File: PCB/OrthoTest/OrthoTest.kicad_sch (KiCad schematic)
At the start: 121 parts, among them SW1 SW_Push, SW10 SW_Push, SW11 SW_Push, SW12 SW_Push, SW13 SW_Push, SW14 SW_Push, SW15 SW_Push, SW16 SW_Push, SW17 SW_Push, SW18 SW_Push, SW19 SW_Push, SW2 SW_Push, SW20 SW_Push, SW21 SW_Push, SW22 SW_Push, SW23 SW_Push, SW24 SW_Push, SW25 SW_Push, SW26 SW_Push, SW27 SW_Push, SW28 SW_Push, SW29 SW_Push, SW3 SW_Push, SW30 SW_Push, SW31 SW_Push, SW32 SW_Push, SW33 SW_Push, SW34 SW_Push, SW35 SW_Push, SW36 SW_Push, SW37 SW_Push, SW38 SW_Push, SW39 SW_Push, SW4 SW_Push, SW40 SW_Push, SW41 SW_Push, SW42 SW_Push, SW43 SW_Push, SW44 SW_Push, SW45 SW_Push, SW46 SW_Push, SW47 SW_Push, SW48 SW_Push, SW49 SW_Push, SW5 SW_Push, SW50 SW_Push, SW51 SW_Push, SW52 SW_Push, SW53 SW_Push, SW54 SW_Push, SW55 SW_Push, SW56 SW_Push, SW57 SW_Push, SW58 SW_Push, SW59 SW_Push, SW6 SW_Push, SW60 SW_Push, SW7 SW_Push, SW8 SW_Push, SW9 SW_Push

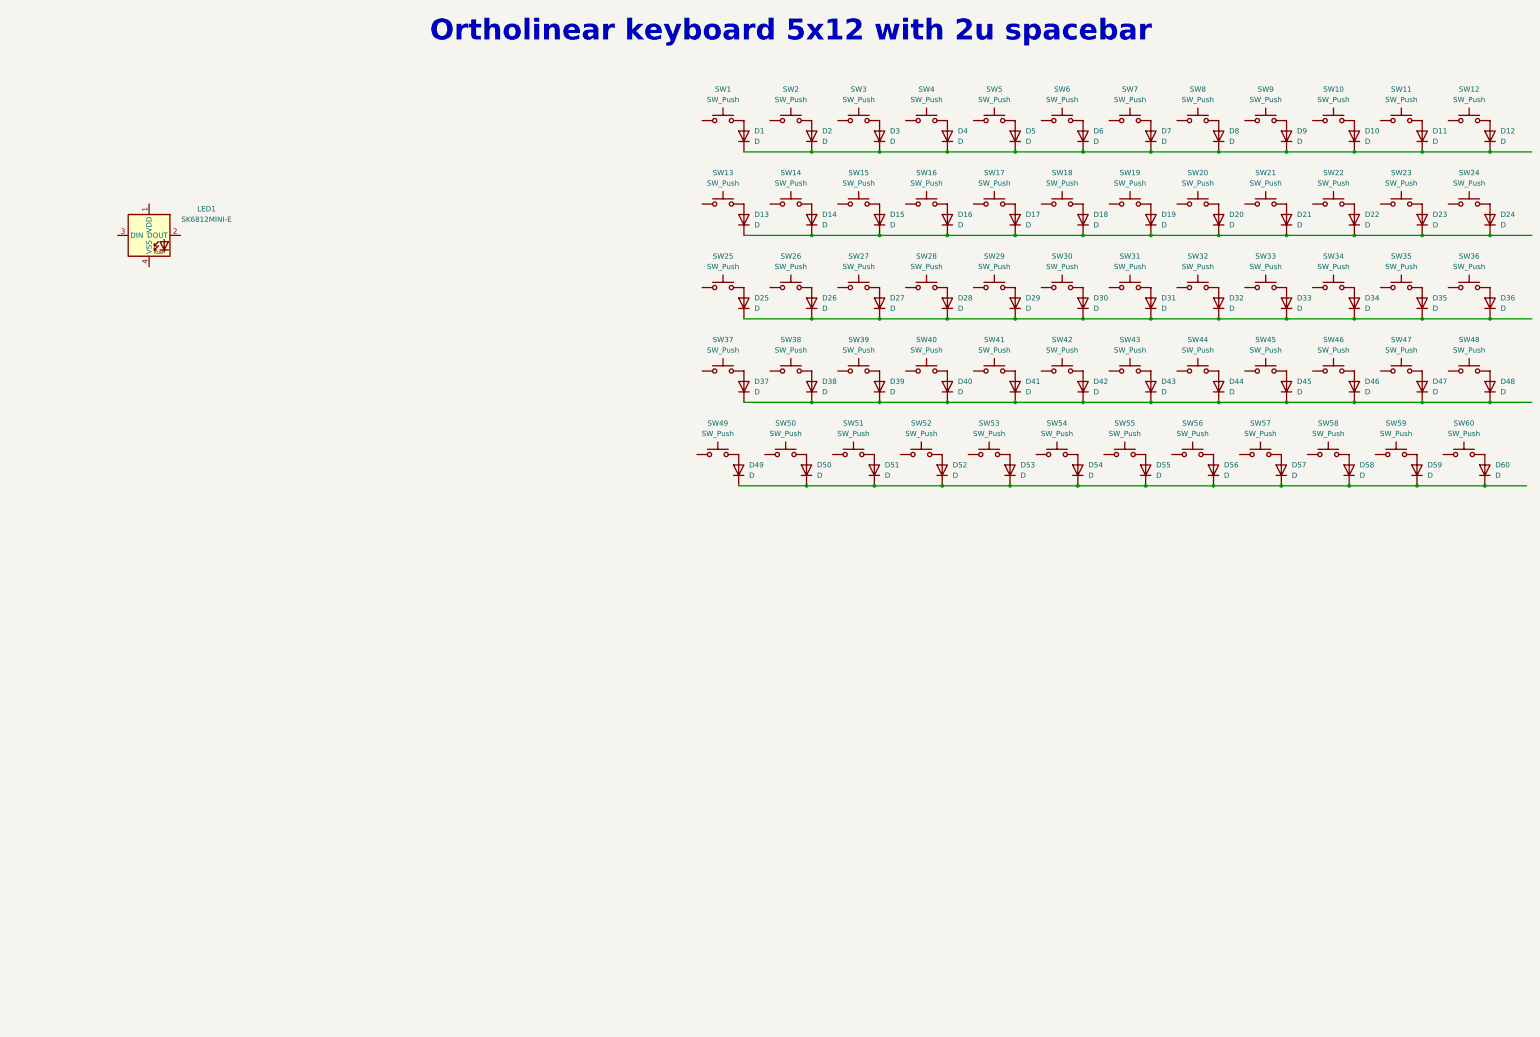
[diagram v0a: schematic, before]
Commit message: worked on it a lil
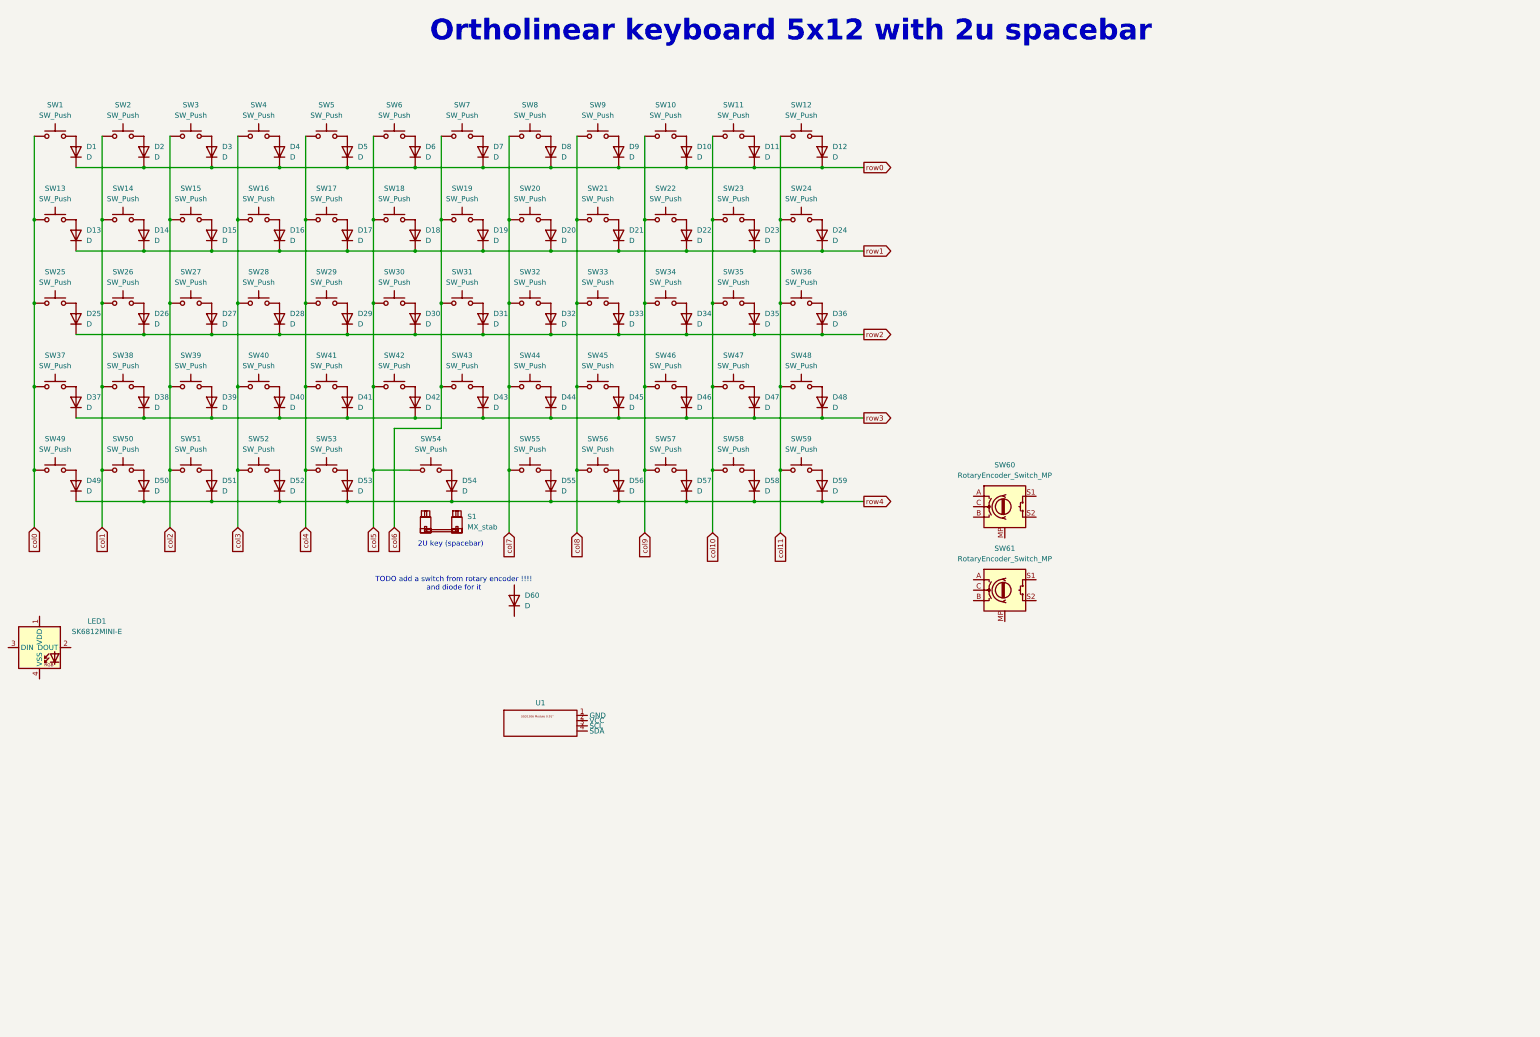
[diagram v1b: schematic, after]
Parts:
- removed SW60: SW_Push, MyKeebLib:SW_Redragon_LowProfile_PCB_1.00u, symbol Switch:SW_Push
- added S1: MX_stab, PCM_marbastlib-mx:STAB_MX_2u, symbol PCM_marbastlib-mx:MX_stab
- added SW60, SW61: RotaryEncoder_Switch_MP, Rotary_Encoder:RotaryEncoder_Alps_EC11E-Switch_Vertical_H20mm, symbol Device:RotaryEncoder_Switch_MP
- added U1: ~, MyKeebLib:SSD1306-0.91-OLED-4pin-128x32, symbol MySymbols:ssd1306
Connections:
- net row1: now reaches D13.1 (K), D14.1 (K), D15.1 (K), D16.1 (K), D17.1 (K), D18.1 (K), D19.1 (K), D20.1 (K), D21.1 (K), D22.1 (K), D23.1 (K), D24.1 (K)
- net row2: now reaches D25.1 (K), D26.1 (K), D27.1 (K), D28.1 (K), D29.1 (K), D30.1 (K), D31.1 (K), D32.1 (K), D33.1 (K), D34.1 (K), D35.1 (K), D36.1 (K)
- net row0: now reaches D1.1 (K), D10.1 (K), D11.1 (K), D12.1 (K), D2.1 (K), D3.1 (K), D4.1 (K), D5.1 (K), D6.1 (K), D7.1 (K), D8.1 (K), D9.1 (K)
- net col10: now reaches SW47.1
- net col10: now also SW11.1, SW23.1, SW35.1, SW58.1
- net row3: now reaches D37.1 (K), D38.1 (K), D39.1 (K), D40.1 (K), D41.1 (K), D42.1 (K), D43.1 (K), D44.1 (K), D45.1 (K), D46.1 (K), D47.1 (K), D48.1 (K)
- net col2: now reaches SW3.1
- net col2: now also SW15.1, SW27.1, SW39.1, SW51.1
- net col0: now reaches SW25.1
- net col0: now also SW1.1, SW13.1, SW37.1, SW49.1
- net col7: now reaches SW8.1
- net col7: now also SW20.1, SW32.1, SW44.1, SW55.1
- net col1: now reaches SW50.1
- net col1: now also SW14.1, SW2.1, SW26.1, SW38.1
- net col5: now reaches SW30.1
- net col5: now also SW18.1, SW42.1, SW54.1, SW6.1
- net col4: now reaches SW41.1
- net col4: now also SW17.1, SW29.1, SW5.1, SW53.1
- net row4: now reaches D49.1 (K), D50.1 (K), D51.1 (K), D52.1 (K), D53.1 (K), D54.1 (K), D55.1 (K), D56.1 (K), D57.1 (K), D58.1 (K), D59.1 (K)
- net row4: no longer D60.1 (K)
- net col3: now reaches SW52.1
- net col3: now also SW16.1, SW28.1, SW4.1, SW40.1
- net col9: now reaches SW22.1
- net col9: now also SW10.1, SW34.1, SW46.1, SW57.1
- net col11: now reaches SW24.1
- net col11: now also SW12.1, SW36.1, SW48.1, SW59.1
- net col8: now reaches SW21.1
- net col8: now also SW33.1, SW45.1, SW56.1, SW9.1
- net col6: now reaches SW19.1
- net col6: now also SW31.1, SW43.1, SW7.1
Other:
- note added: "2U key (spacebar)"
- note added: "TODO add a switch from rotary encoder !!!! and diode for it"
- moved on the sheet: D1, D10, D11, D12, D13, D14, D15, D16, D17, D18, D19, D2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

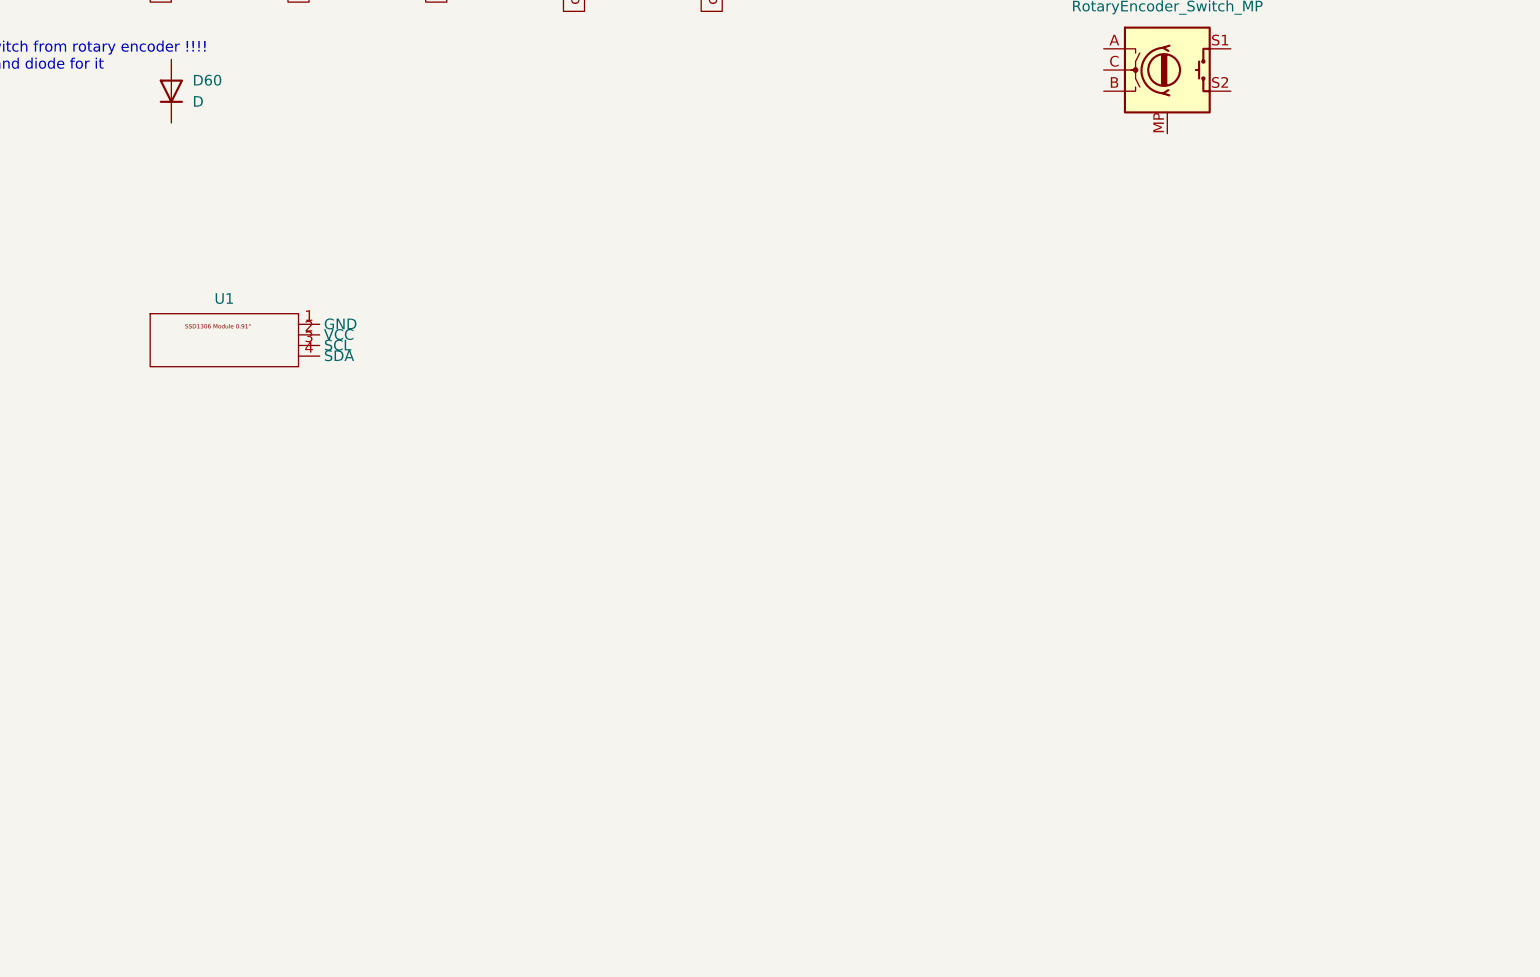
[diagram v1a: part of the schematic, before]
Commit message: worked a lil on it
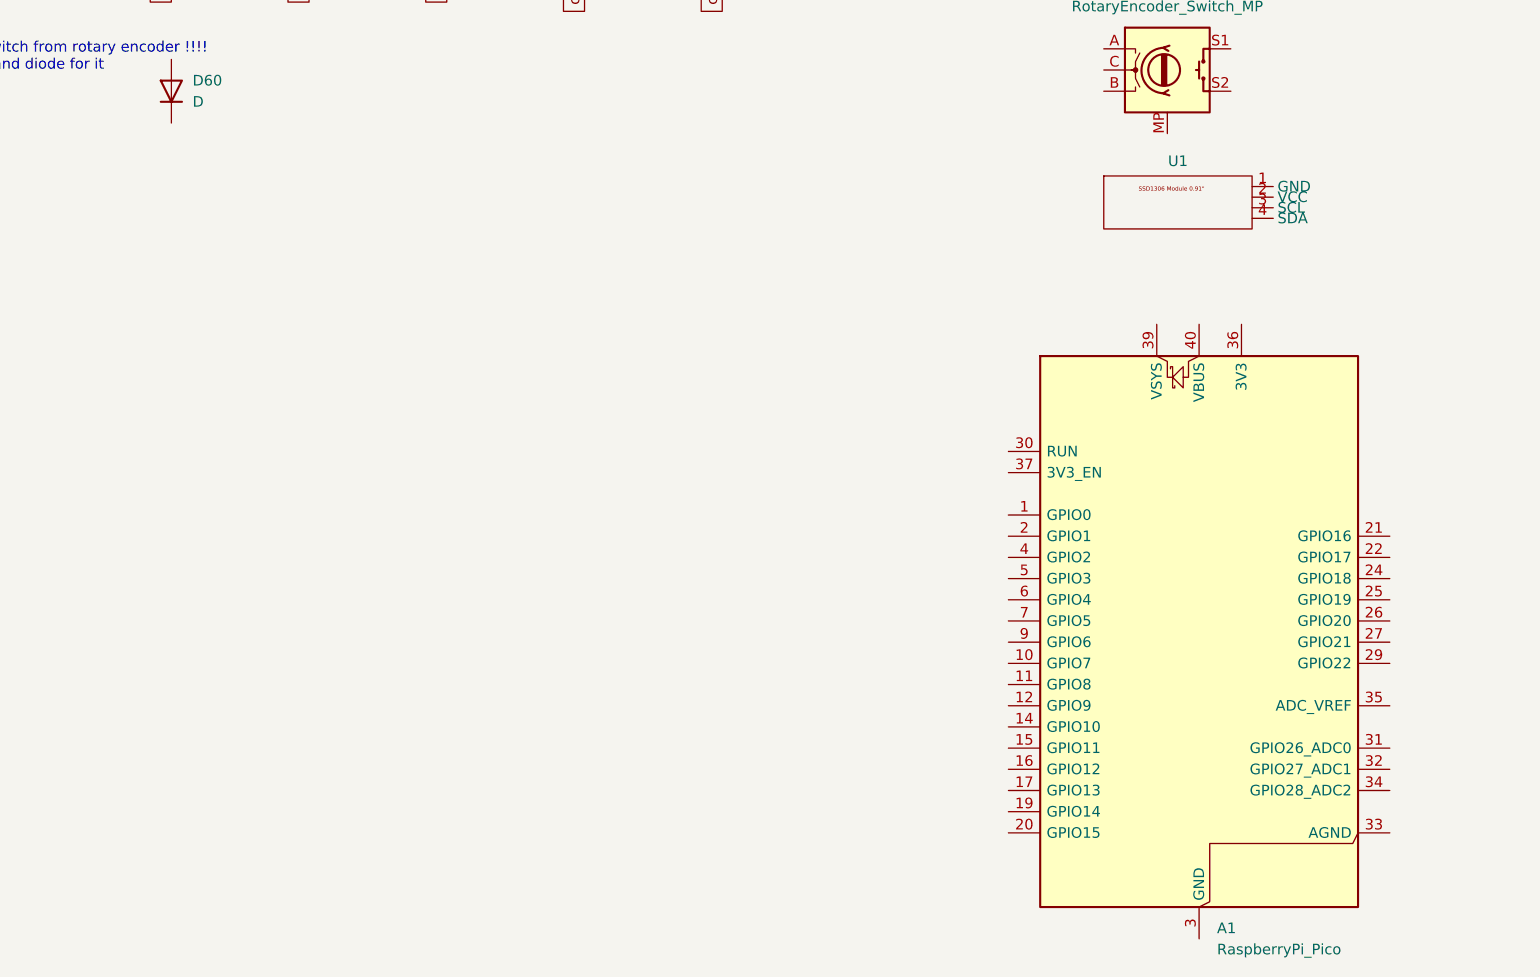
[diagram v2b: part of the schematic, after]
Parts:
- added A1: RaspberryPi_Pico, Module:RaspberryPi_Pico_Common_SMD, symbol MCU_Module:RaspberryPi_Pico
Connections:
- new net: A1.13 (GND), A1.18 (GND), A1.23 (GND), A1.28 (GND), A1.3 (GND), A1.38 (GND), A1.8 (GND)
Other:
- moved on the sheet: U1
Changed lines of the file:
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@@
 	(symbol
 		(lib_id "MySymbols:ssd1306")
-		(at 151.13 189.23 0)
+		(at 265.43 172.72 0)
 		(unit 1)
 		(exclude_from_sim no)
@@
 		(dnp no)
 		(property "Reference" "U1"
-			(at 151.13 188.722 0)
+			(at 265.43 172.212 0)
 			(effects
 				(font
@@
 		)
 		(property "Value" "~"
-			(at 152.4 189.23 0)
+			(at 266.7 172.72 0)
 			(effects
 				(font
@@
 		)
 		(property "Footprint" "MyKeebLib:SSD1306-0.91-OLED-4pin-128x32"
-			(at 151.13 189.23 0)
+			(at 265.43 172.72 0)
 			(effects
 				(font
@@
 		)
 		(property "Datasheet" ""
-			(at 151.13 189.23 0)
+			(at 265.43 172.72 0)
 			(effects
 				(font
@@
 		)
 		(property "Description" ""
-			(at 151.13 189.23 0)
+			(at 265.43 172.72 0)
 			(effects
 				(font
@@
 					(unit 1)
 				)
+			)
+		)
+	)
+	(symbol
+		(lib_id "MCU_Module:RaspberryPi_Pico")
+		(at 267.97 229.87 0)
+		(unit 1)
+		(exclude_from_sim no)
+		(in_bom yes)
+		(on_board yes)
+		(dnp no)
+		(fields_autoplaced yes)
+		(property "Reference" "A1"
+			(at 270.1133 264.16 0)
+			(effects
+				(font
+					(size 1.27 1.27)
+				)
+				(justify left)
+			)
+		)
+		(property "Value" "RaspberryPi_Pico"
+			(at 270.1133 266.7 0)
+			(effects
+				(font
+					(size 1.27 1.27)
+				)
+				(justify left)
+			)
+		)
+		(property "Footprint" "Module:RaspberryPi_Pico_Common_SMD"
+			(at 267.97 276.86 0)
+			(effects
+				(font
+					(size 1.27 1.27)
+				)
+				(hide yes)
+			)
+		)
+		(property "Datasheet" "https://datasheets.raspberrypi.com/pico/pico-datasheet.pdf"
+			(at 267.97 279.4 0)
+			(effects
+				(font
+					(size 1.27 1.27)
+				)
+				(hide yes)
+			)
+		)
+		(property "Description" "Versatile and inexpensive microcontroller module powered by RP2040 dual-core Arm Cortex-M0+ processor up to 133 MHz, 264kB SRAM, 2MB QSPI flash; also supports Raspberry Pi Pico 2"
+			(at 267.97 281.94 0)
+			(effects
+				(font
+					(size 1.27 1.27)
+				)
+				(hide yes)
+			)
+		)
+		(pin "37"
+		)
+		(pin "17"
+		)
+		(pin "19"
+		)
+		(pin "30"
+		)
+		(pin "1"
+		)
+		(pin "2"
+		)
+		(pin "4"
+		)
+		(pin "5"
+		)
+		(pin "6"
+		)
+		(pin "10"
+		)
+		(pin "9"
+		)
+		(pin "11"
+		)
+		(pin "14"
+		)
+		(pin "15"
+		)
+		(pin "7"
+		)
+		(pin "12"
+		)
+		(pin "16"
+		)
+		(pin "22"
+		)
+		(pin "23"
+		)
+		(pin "28"
+		)
+		(pin "38"
+		)
+		(pin "24"
+		)
+		(pin "31"
+		)
+		(pin "8"
+		)
+		(pin "20"
+		)
+		(pin "25"
+		)
+		(pin "13"
+		)
+		(pin "39"
+		)
+		(pin "18"
+		)
+		(pin "27"
+		)
+		(pin "21"
+		)
+		(pin "35"
+		)
+		(pin "40"
+		)
+		(pin "34"
+		)
+		(pin "36"
+		)
+		(pin "33"
+		)
+		(pin "3"
+		)
+		(pin "26"
+		)
+		(pin "32"
+		)
+		(pin "29"
+		)
+		(instances
+			(project ""
+				(path "/63f5a0a7-4058-42ed-a215-6578acb070e1"
+					(reference "A1")
+					(unit 1)
+				)
